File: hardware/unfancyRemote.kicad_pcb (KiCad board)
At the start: 2 copper layers, 27.7 x 59.2 mm, 41 parts, among them J1 Arduino Analog, J2 Arduino Digital, J3 HALL1, J4 HALL2, J5 PPM, J6 VIN, J7 VBAT, J8 Motor, J9 Extra analog 1, Q1 AO3401A, Q2 MMBT3904, Q3 MMBT3904, SW1 SW_Push, U1 E28-2G4M12S

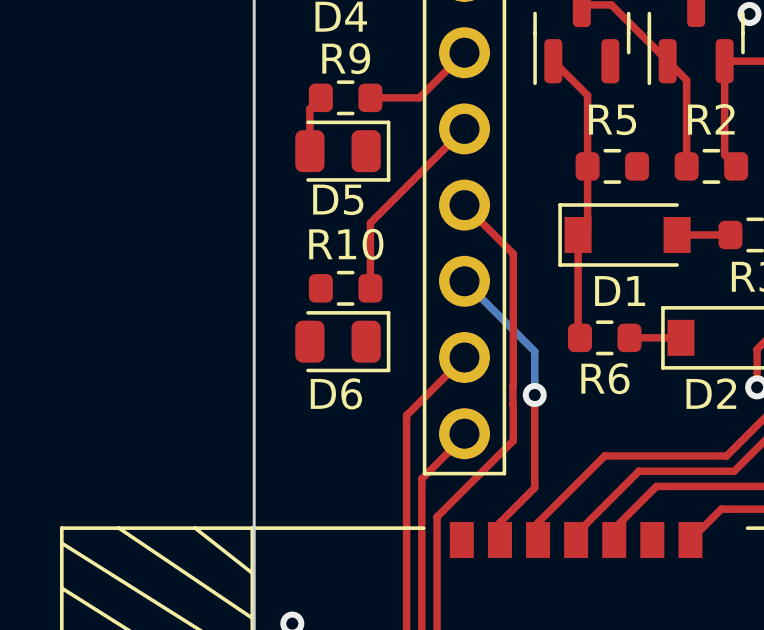
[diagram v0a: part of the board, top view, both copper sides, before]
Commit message: Software v1.0 for rx and tx
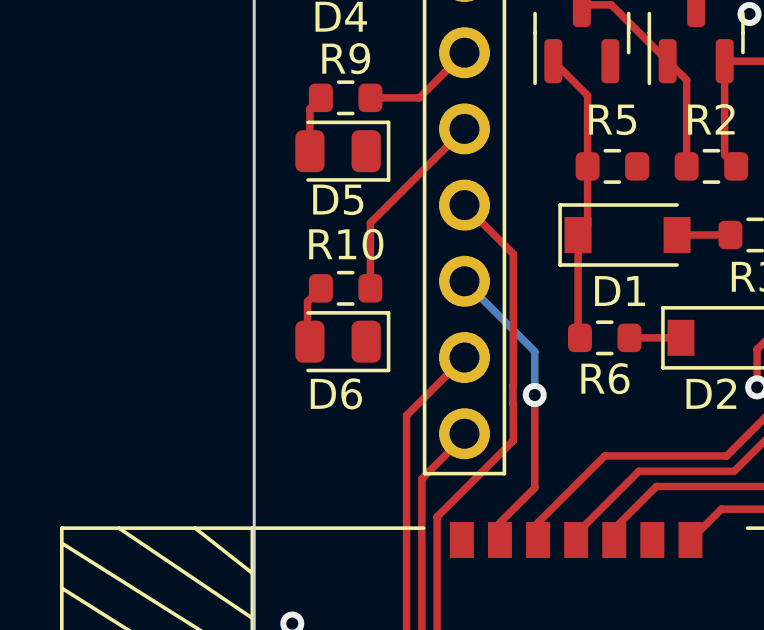
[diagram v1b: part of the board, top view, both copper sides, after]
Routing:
- net Net-(D6-Pad2): track 0.00 -> 1.99 mm
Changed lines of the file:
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@@
   (segment (start 121.2365 89.662) (end 121.2365 88.2505) (width 0.25) (layer "F.Cu") (net 26))
   (segment (start 121.2365 88.2505) (end 121.603 87.884) (width 0.25) (layer "F.Cu") (net 26))
+  (segment (start 121.603 94.234) (end 121.158 94.679) (width 0.25) (layer "F.Cu") (net 27))
+  (segment (start 121.158 94.679) (end 121.158 95.9335) (width 0.25) (layer "F.Cu") (net 27))
+  (segment (start 121.158 95.9335) (end 121.2365 96.012) (width 0.25) (layer "F.Cu") (net 27))
   (segment (start 123.253 92.057) (end 126.39 88.92) (width 0.25) (layer "F.Cu") (net 28))
   (segment (start 123.253 94.234) (end 123.253 92.057) (width 0.25) (layer "F.Cu") (net 28))
